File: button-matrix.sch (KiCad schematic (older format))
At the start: 79 parts, among them SW301 TL1105T, SW302 TL1105T, SW303 TL1105T, SW304 TL1105T, SW305 TL1105T, SW309 TL1105T, SW310 TL1105T, SW311 TL1105T, SW312 TL1105T, SW313 TL1105T, SW314 TL1105T, SW315 TL1105T, SW316 TL1105T, SW317 TL1105T, SW318 TL1105T, SW319 TL1105T, SW320 TL1105T, SW321 TL1105T, SW322 TL1105T, SW323 TL1105T, SW324 TL1105T, SW325 TL1105T, SW326 TL1105T, SW327 TL1105T, SW328 TL1105T, SW329 TL1105T, SW330 TL1105T, SW331 TL1105T, SW332 TL1105T, SW333 TL1105T, SW334 TL1105T, SW335 TL1105T, SW336 TL1105T, SW337 TL1105T, SW338 TL1105T, SW339 TL1105T, SW340 TL1105T

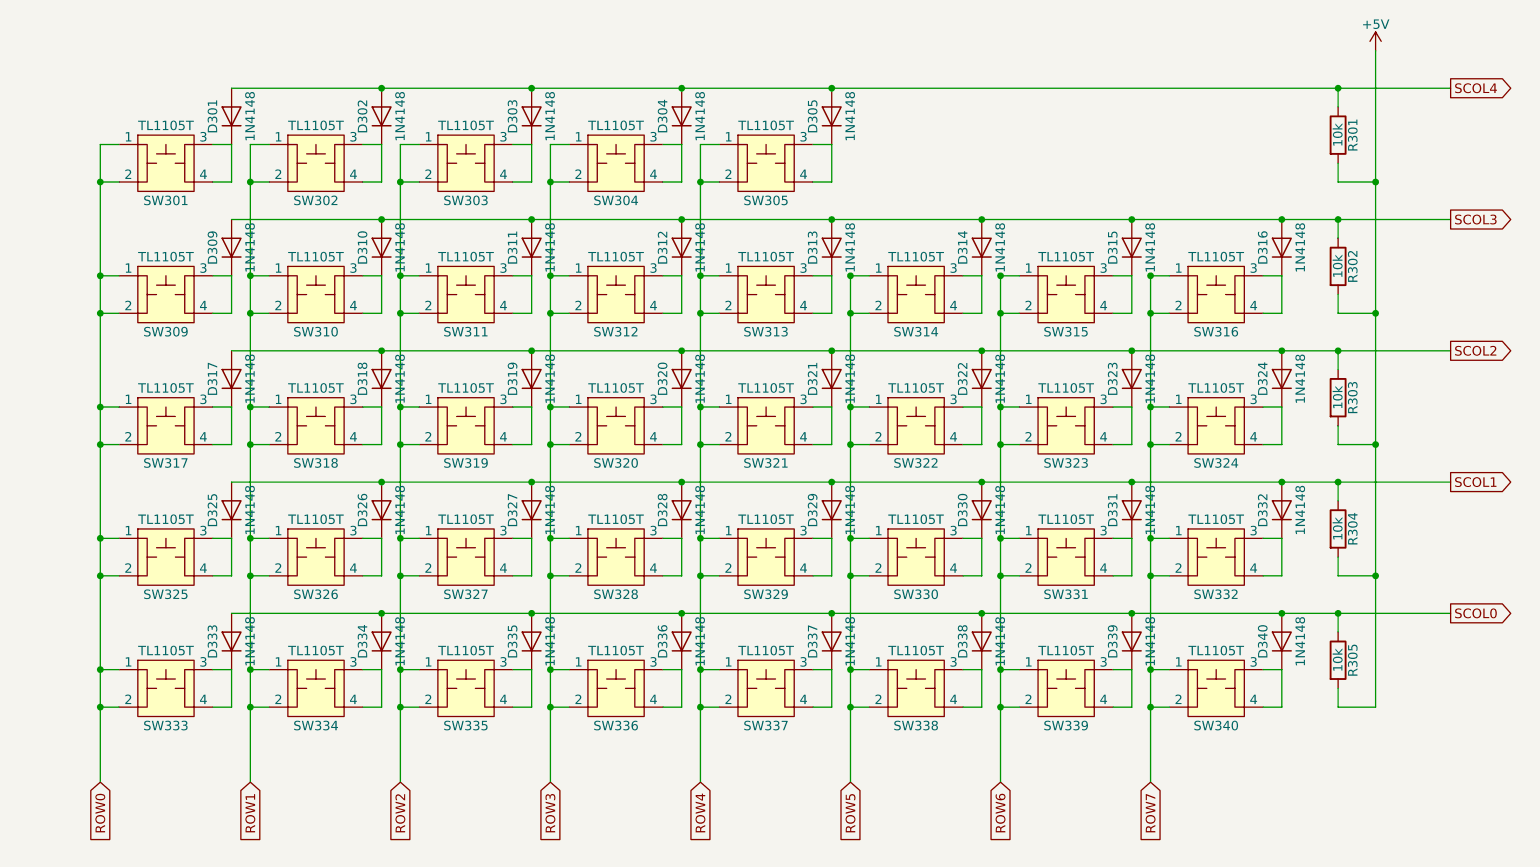
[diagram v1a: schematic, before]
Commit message: work in progress
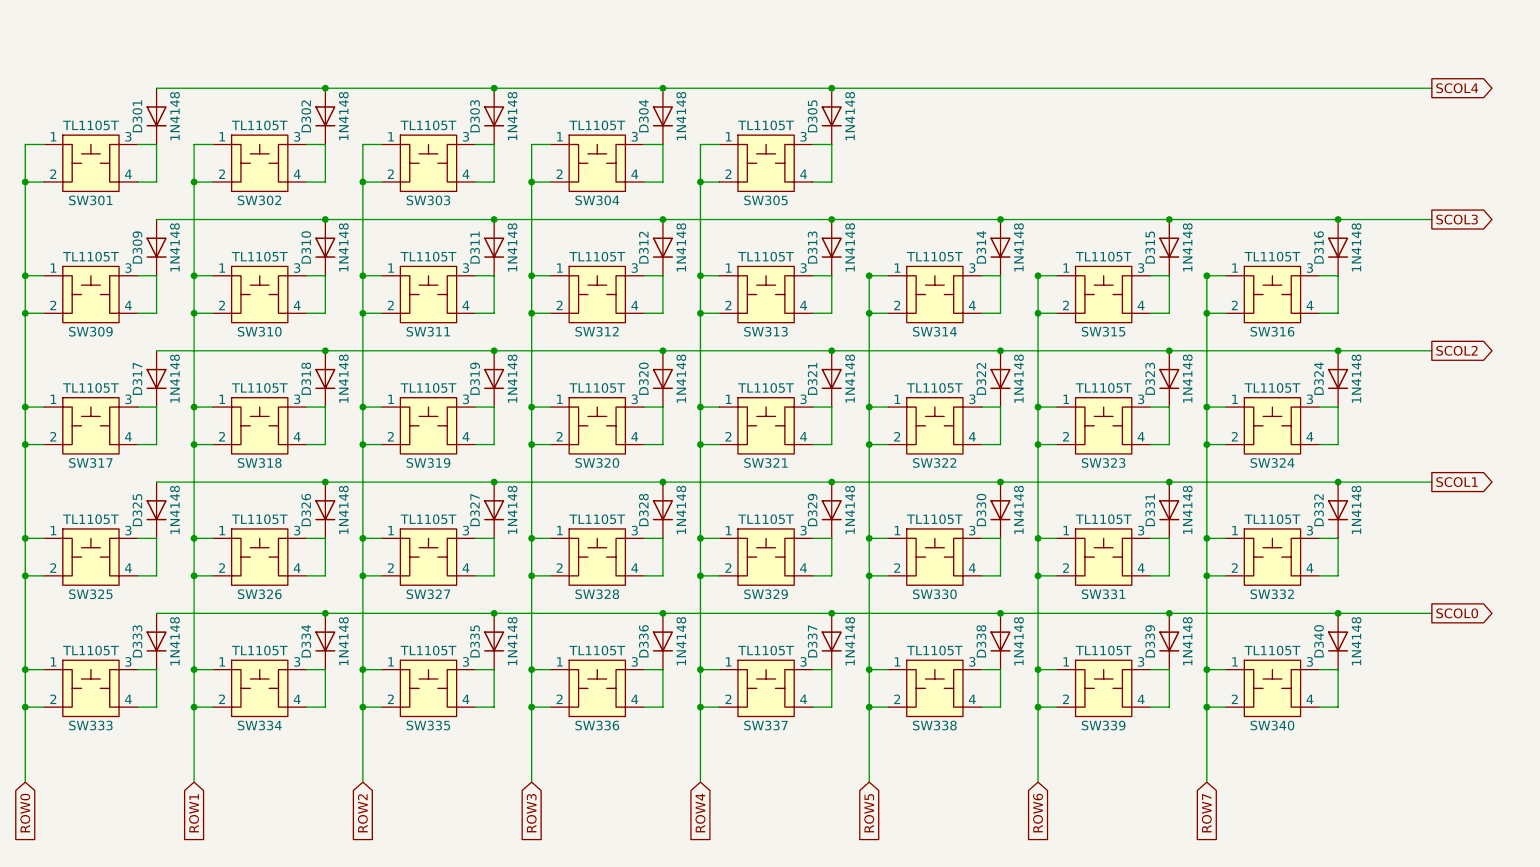
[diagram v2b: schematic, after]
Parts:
- removed R301, R302, R303, R304, R305: 10k, Resistors_SMD:R_0603, symbol R
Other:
- moved on the sheet: D301, D302, D303, D304, D309, D310, D311, D312, D314, D315, D316, D317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

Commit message: cleanup
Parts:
- D301, D302, D303, D304, D305, D309, D310, D311, D312, D313, D314, D315, D316, D317, D318, D319, D320, D321, D322, D323, D324, D325, D326, D327, D328, D329, D330, D331, D332, D333, D334, D335, D336, D337, D338, D339, D340: footprint Diodes_SMD:D_SOD-123 -> w_diode:D_SOD-123
